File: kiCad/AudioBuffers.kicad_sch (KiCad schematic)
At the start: 35 parts, among them U1 MCP6024

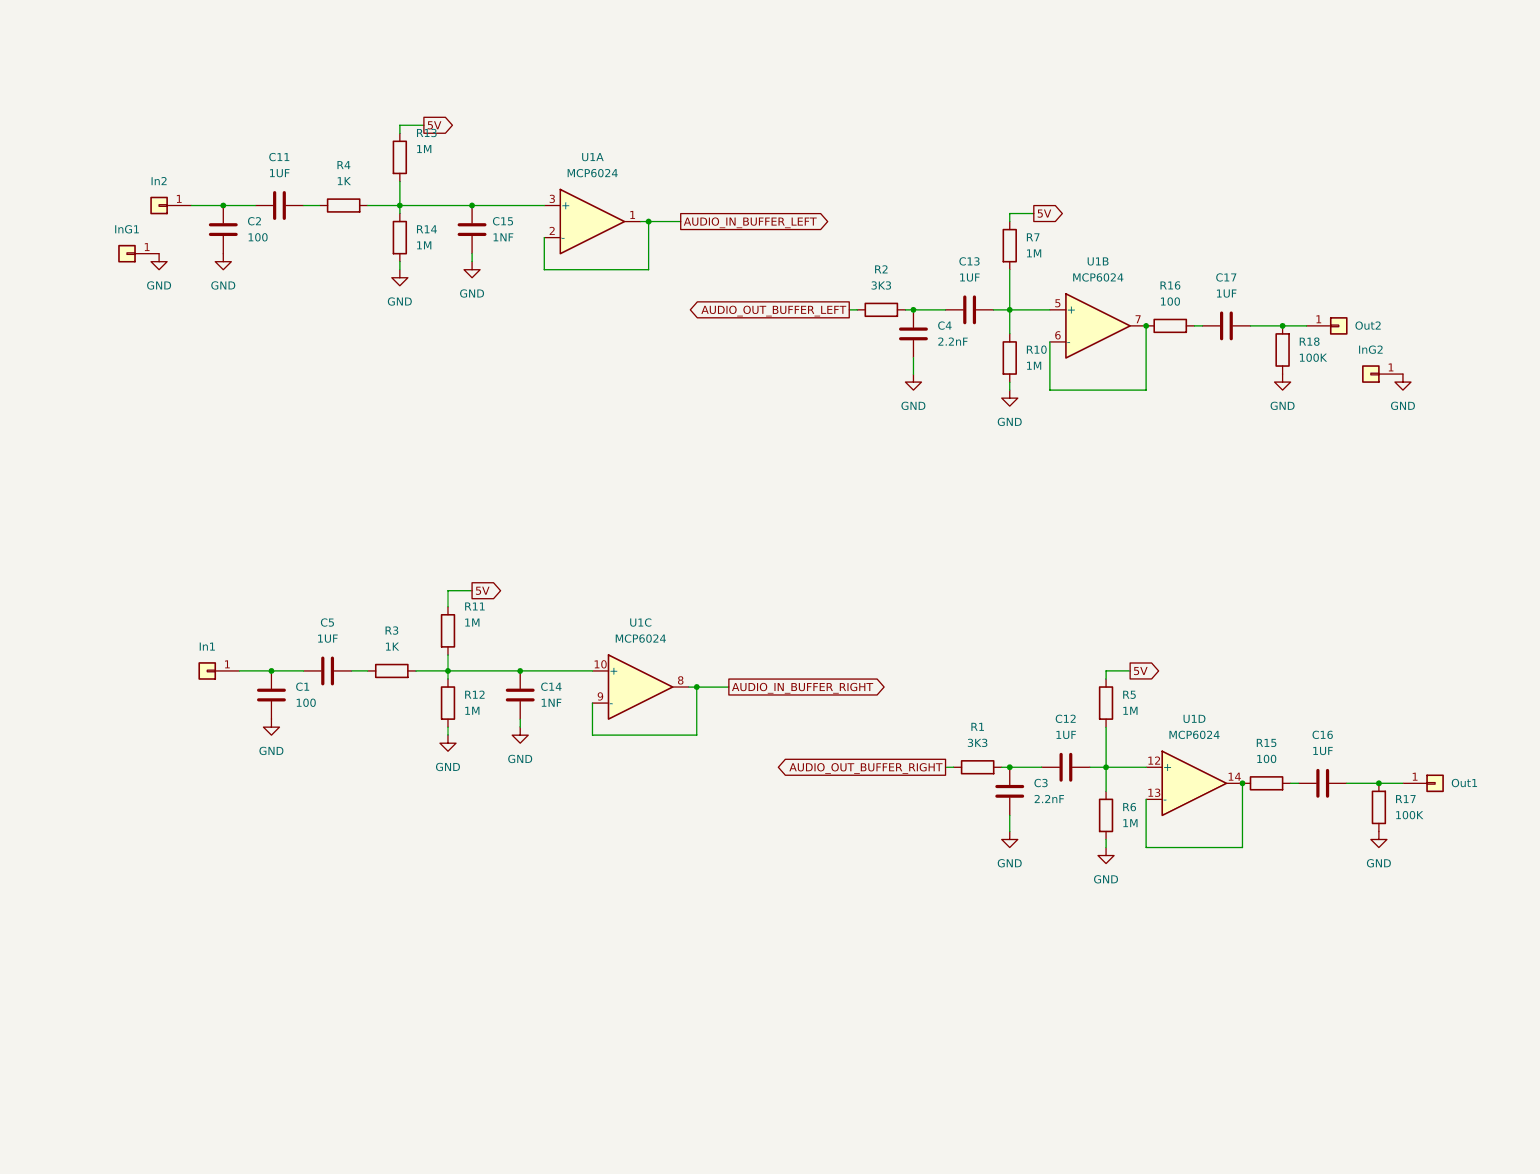
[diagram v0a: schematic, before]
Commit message: Updated kiCad Project
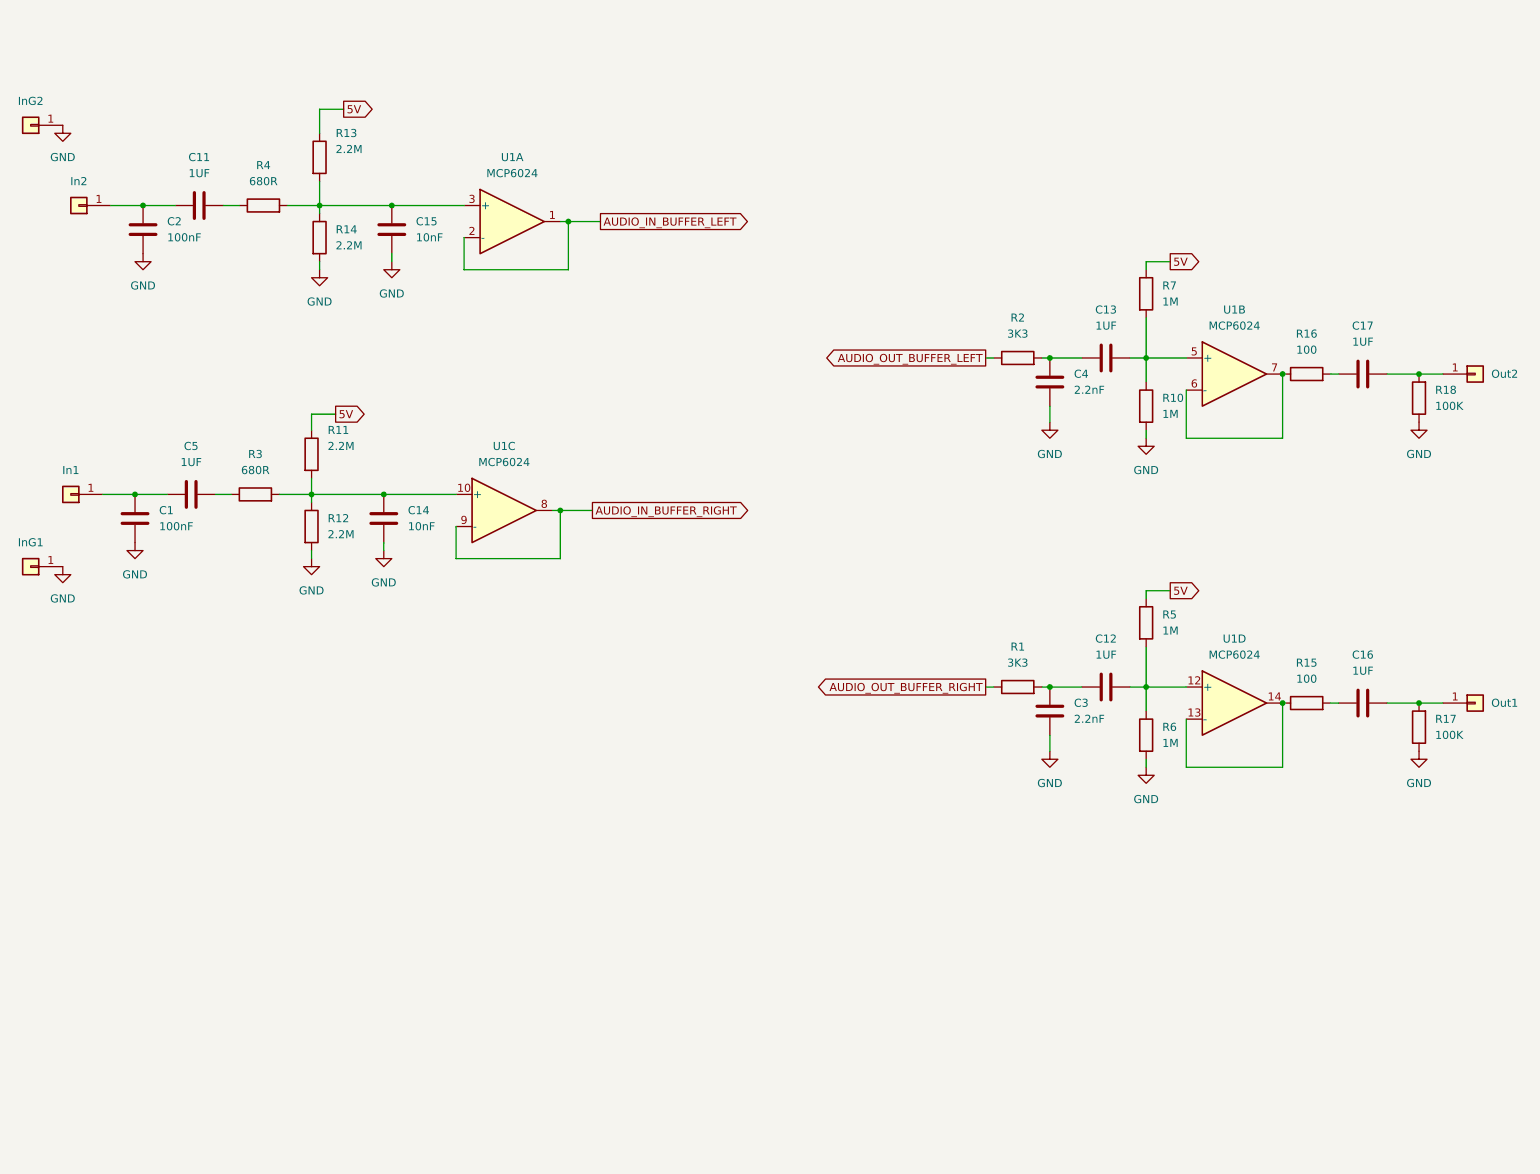
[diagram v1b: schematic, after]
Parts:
- C1, C2: value 100 -> 100nF
- C14, C15: value 1NF -> 10nF
- R11, R12, R13, R14: value 1M -> 2.2M
- R3, R4: value 1K -> 680R
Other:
- moved on the sheet: C1, C11, C12, C13, C14, C15, C16, C17, C2, C3, C4, C5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

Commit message: Lots of stuff
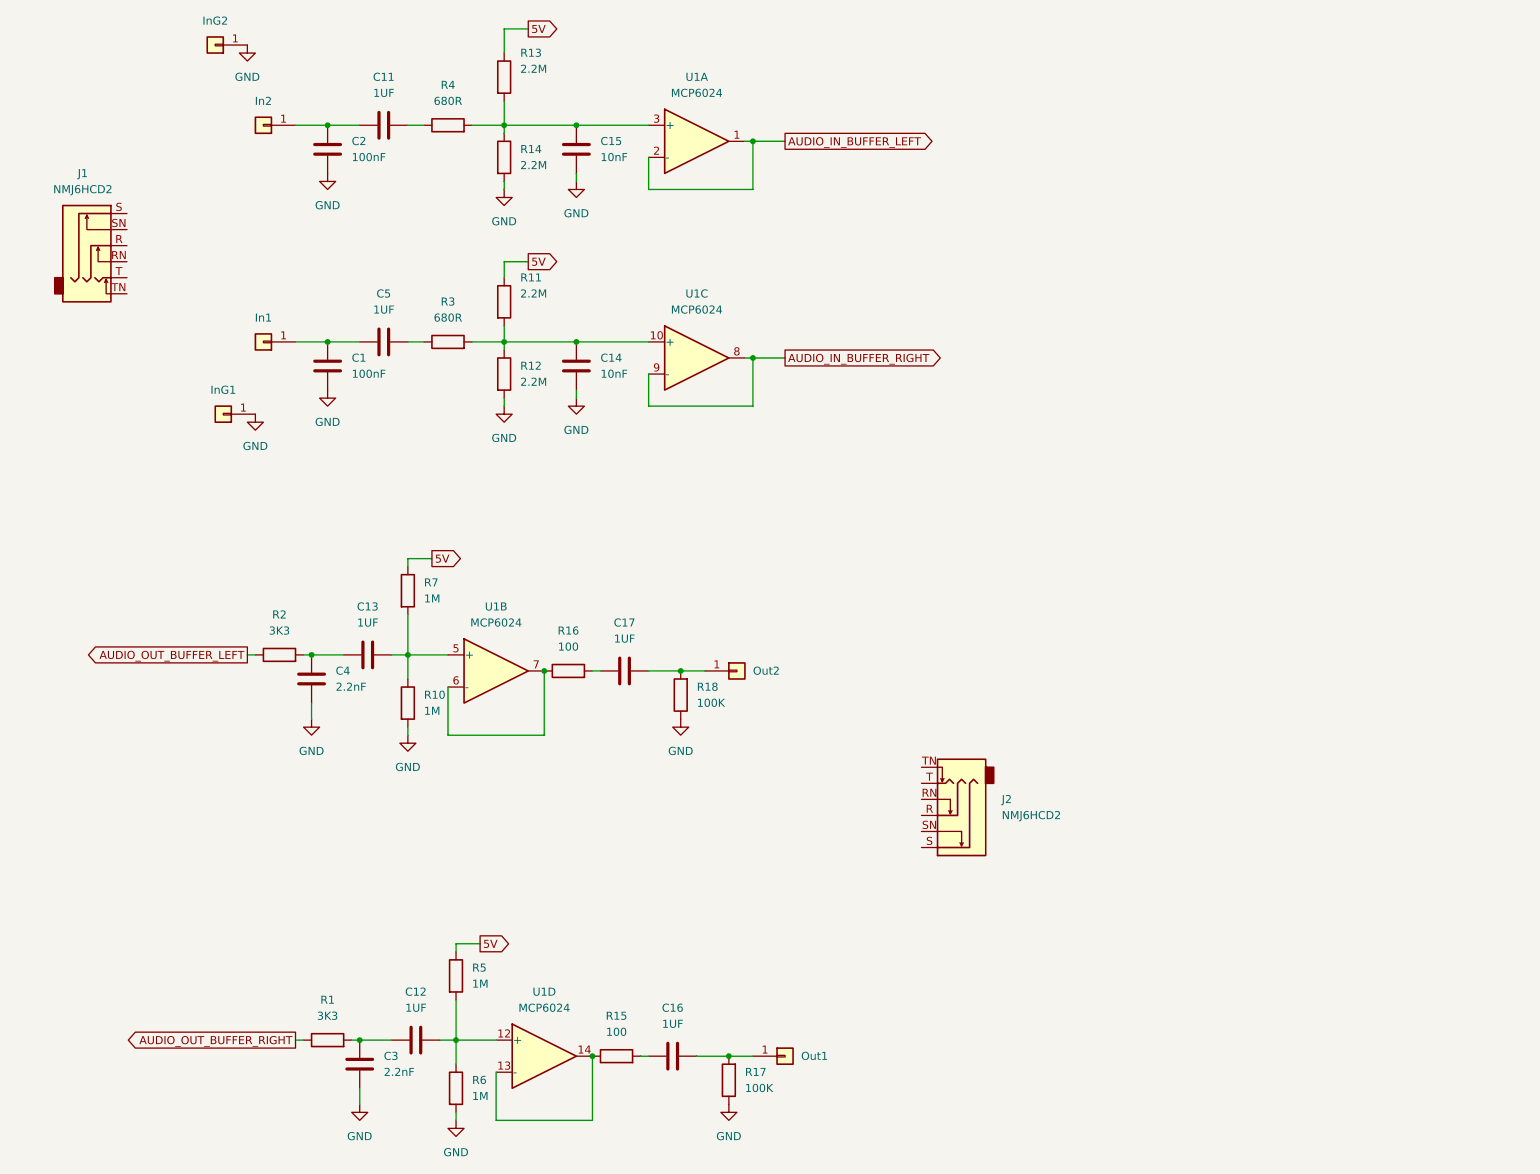
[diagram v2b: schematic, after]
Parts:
- added J1, J2: NMJ6HCD2, Connector_Audio:Jack_6.35mm_Neutrik_NMJ6HCD2_Horizontal, symbol Connector_Audio:NMJ6HCD2
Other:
- moved on the sheet: C1, C11, C12, C13, C14, C15, C16, C17, C2, C3, C4, C5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
